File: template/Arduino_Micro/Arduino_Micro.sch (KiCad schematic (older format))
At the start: 6 parts, among them P1 Digital, P2 Analog, P3 CONN_1, P4 CONN_1, P5 CONN_1, P6 CONN_1

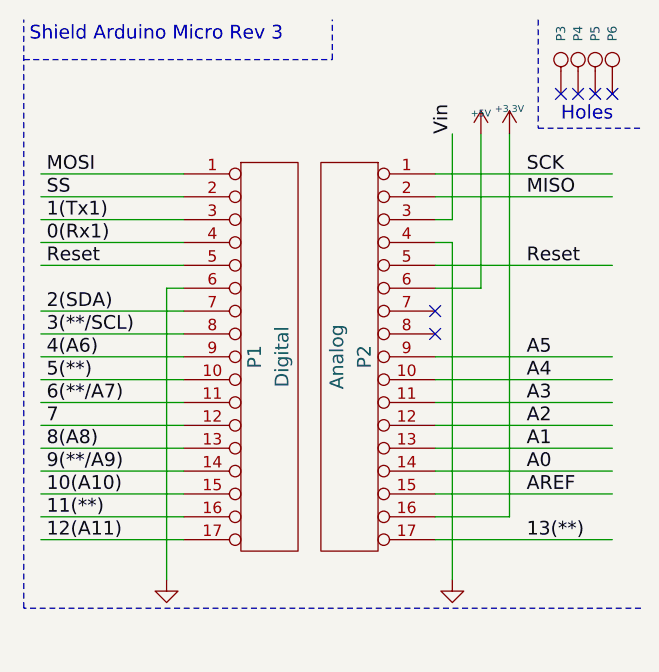
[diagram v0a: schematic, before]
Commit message: rebuilt shematic and fix librairie
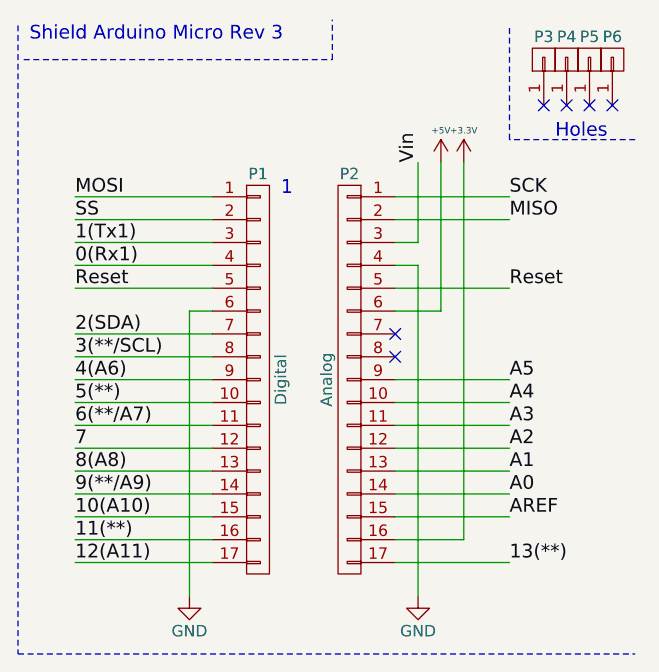
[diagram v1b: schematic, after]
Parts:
- removed P1: Digital, Socket_Arduino_Micro:Socket_Strip_Arduino_1x17, symbol CONN_17
- removed P2: Analog, Socket_Arduino_Micro:Socket_Strip_Arduino_1x17, symbol CONN_17
- removed P3, P4, P5, P6: CONN_1, Socket_Arduino_Micro:1pin_Micro, symbol CONN_1
- added P1: Digital, Socket_Arduino_Micro:Socket_Strip_Arduino_1x17, symbol CONN_01X17
- added P2: Analog, Socket_Arduino_Micro:Socket_Strip_Arduino_1x17, symbol CONN_01X17
- added P3, P4, P5, P6: CONN_01X01, Socket_Arduino_Micro:1pin_Micro, symbol CONN_01X01
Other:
- note added: "1"
